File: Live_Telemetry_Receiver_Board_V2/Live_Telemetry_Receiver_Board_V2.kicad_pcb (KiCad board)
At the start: 2 copper layers, 53.5 x 69.5 mm, 8 parts, among them CN1 NUCLEO-L432KC, U2 XBP9B-DPST-001

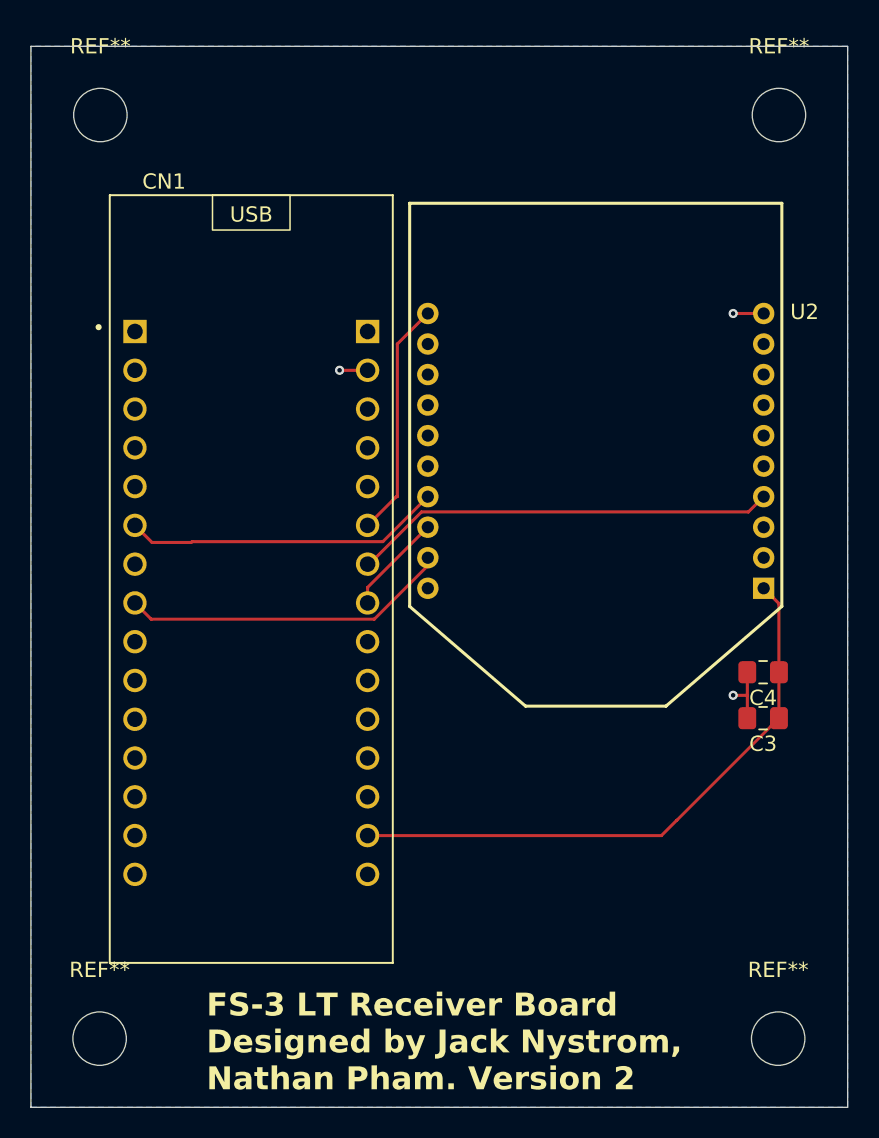
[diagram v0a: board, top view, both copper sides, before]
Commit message: update pcb dimensions
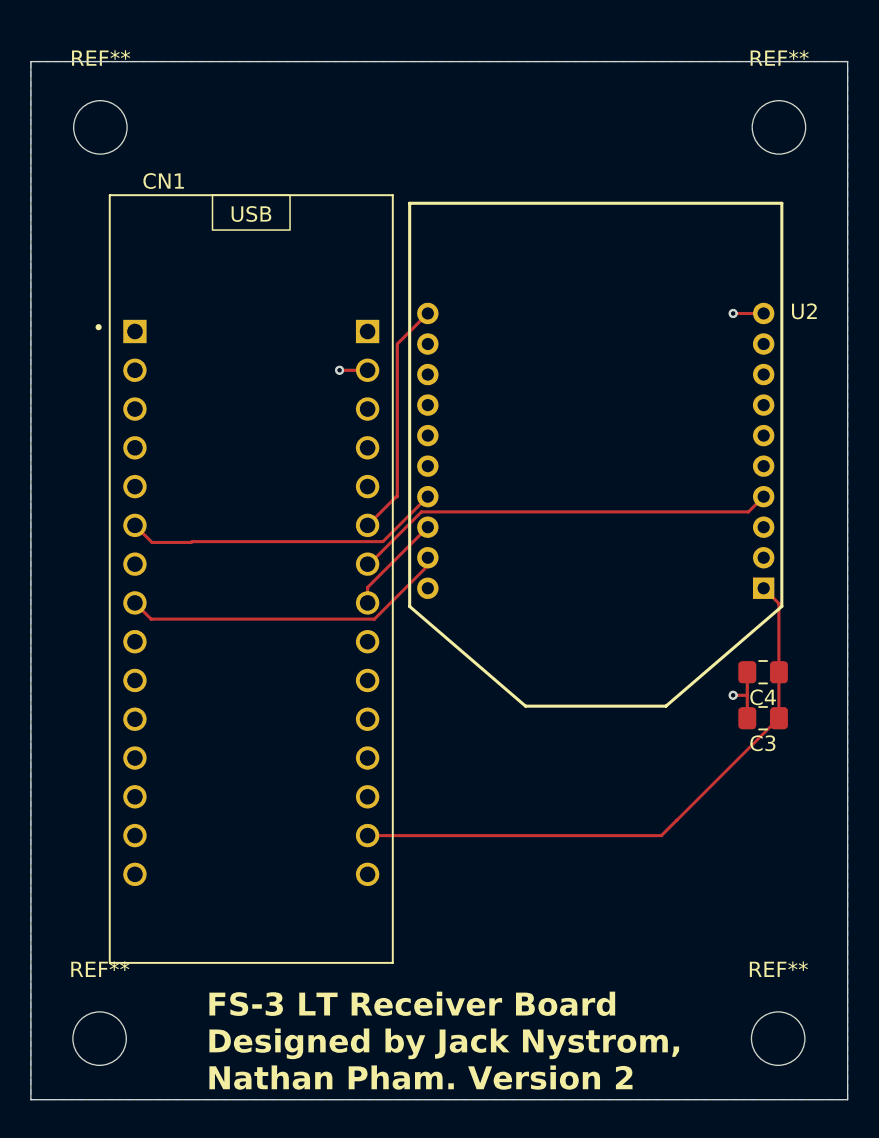
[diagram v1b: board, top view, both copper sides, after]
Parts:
- moved REF** 0.81 mm to (108.5, 44.3)
- moved REF** 0.81 mm to (64.0, 44.3)
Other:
- board size 53.5 x 69.5 mm -> 53.5 x 68 mm
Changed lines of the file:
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@@
 		(descr "General ISM < 1GHz Transceiver Module 900MHz")
 		(property "Reference" "U2"
-			(at -13.67664 9.3535 360)
+			(at -13.67664 9.3535 0)
 			(layer "F.SilkS")
 			(effects
@@
 		)
 		(property "Value" "XBP9B-DPST-001"
-			(at 13.62904 -4.14932 360)
+			(at 13.62904 -4.14932 0)
 			(layer "F.Fab")
 			(effects
@@
 		)
 		(property "Footprint" "FS_3_Global_Footprint_Library:XBP9B-DPST-001"
-			(at 0 0 360)
+			(at 0 0 0)
 			(layer "F.Fab")
 			(hide yes)
@@
 		)
 		(property "Datasheet" "https://www.digi.com/resources/documentation/digidocs/pdfs/90002173.pdf"
-			(at 0 0 360)
+			(at 0 0 0)
 			(layer "F.Fab")
 			(hide yes)
@@
 		)
 		(property "Description" "General ISM < 1GHz Transceiver Module 900MHz"
-			(at 0 0 360)
+			(at 0 0 0)
 			(layer "F.Fab")
 			(hide yes)
@@
 	(footprint "MountingHole:MountingHole_3.5mm"
 		(layer "F.Cu")
-		(at 108.5 43.5)
+		(at 108.5 44.31)
 		(descr "Mounting Hole 3.5mm, no annular")
 		(tags "mounting hole 3.5mm no annular")
@@
 		(tags "capacitor handsolder")
 		(property "Reference" "C4"
-			(at 0 -1.68 360)
+			(at 0 -1.68 0)
 			(layer "F.SilkS")
 			(effects
@@
 		)
 		(property "Value" "47 pF"
-			(at 0 1.68 360)
+			(at 0 1.68 0)
 			(layer "F.Fab")
 			(effects
@@
 		)
 		(fp_text user "${REFERENCE}"
-			(at 0 0 360)
+			(at 0 0 0)
 			(layer "F.Fab")
 			(effects
@@
 	(footprint "MountingHole:MountingHole_3.5mm"
 		(layer "F.Cu")
-		(at 64.05 43.5)
+		(at 64.05 44.31)
 		(descr "Mounting Hole 3.5mm, no annular")
 		(tags "mounting hole 3.5mm no annular")
@@
 		(tags "capacitor handsolder")
 		(property "Reference" "C3"
-			(at 0 -1.68 360)
+			(at 0 -1.68 0)
 			(layer "F.SilkS")
 			(effects
@@
 		)
 		(property "Value" "1.0 uF"
-			(at 0 1.68 360)
+			(at 0 1.68 0)
 			(layer "F.Fab")
 			(effects
@@
 		)
 		(fp_text user "${REFERENCE}"
-			(at 0 0 360)
+			(at 0 0 0)
 			(layer "F.Fab")
 			(effects
@@
 	)
 	(gr_rect
-		(start 59.5 39)
-		(end 113 108.5)
+		(start 59.5 40)
+		(end 113 108)
 		(stroke
 			(width 0.05)
@@
 	(dimension
 		(type aligned)
+		(layer "Edge.Cuts")
+		(pts
+			(xy 64 104) (xy 64.05 44.31)
+		)
+		(height -8.658439)
+		(gr_text "2.3500 in"
+			(at 54.216564 74.146784 89.95200556)
+			(layer "Edge.Cuts")
+			(effects
+				(font
+					(size 1 1)
+					(thickness 0.15)
+				)
+			)
+		)
+		(format
+			(prefix "")
+			(suffix "")
+			(units 0)
+			(units_format 1)
+			(precision 4)
+		)
+		(style
+			(thickness 0.05)
+			(arrow_length 1.27)
+			(text_position_mode 0)
+			(extension_height 0.58642)
+			(extension_offset 0.5) keep_text_aligned)
+	)
+	(dimension
+		(type aligned)
 		(layer "F.Fab")
 		(pts
@@
 		(polygon
 			(pts
-				(xy 59.5 39) (xy 59.5 108.5) (xy 113 108.5) (xy 113 39)
-			)
-		)
+				(xy 59.5 40) (xy 59.5 108) (xy 113 108) (xy 113 40)
+			)
+		)
